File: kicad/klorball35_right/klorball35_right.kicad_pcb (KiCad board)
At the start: 2 copper layers, 138.1 x 106.1 mm, 26 parts, among them J1 TRRS, J2 Conn_01x07, SW1 SW_Push, SW11 SW_Push, SW12 SW_Push, SW13 SW_Push, SW14 SW_Push, SW15 SW_Push, SW16 SW_Push, SW17 SW_Push, SW18 SW_Push, SW2 SW_Push, SW3 SW_Push, SW4 SW_Push, SW5 SW_Push, SW6 SW_Push, SW7 SW_Push, SW8 SW_Push, SW9 SW_Push, U1 Helios

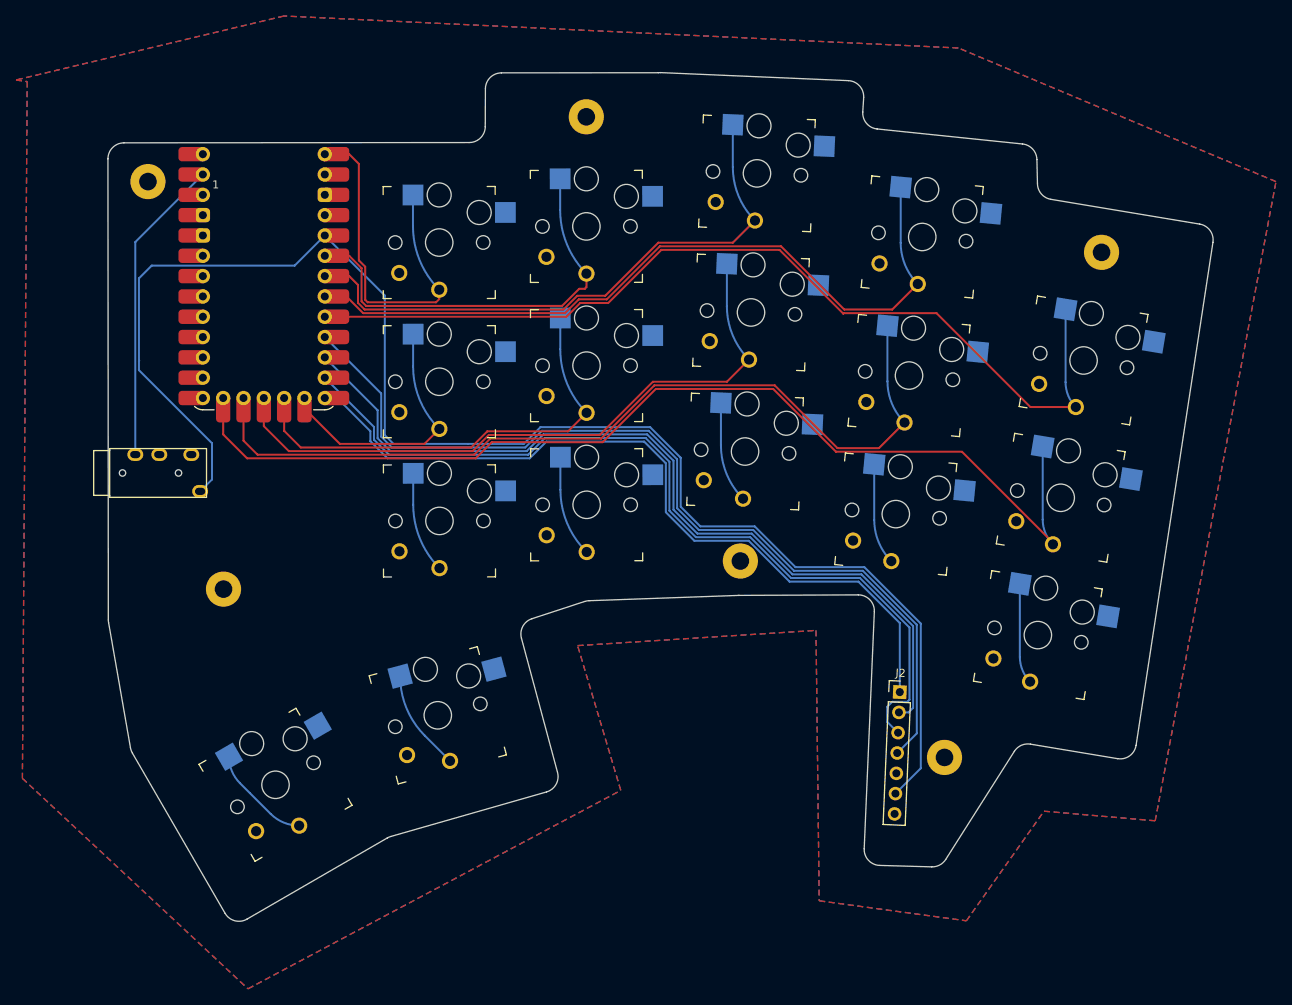
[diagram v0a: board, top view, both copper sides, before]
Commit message: finishing right, start of gerbers
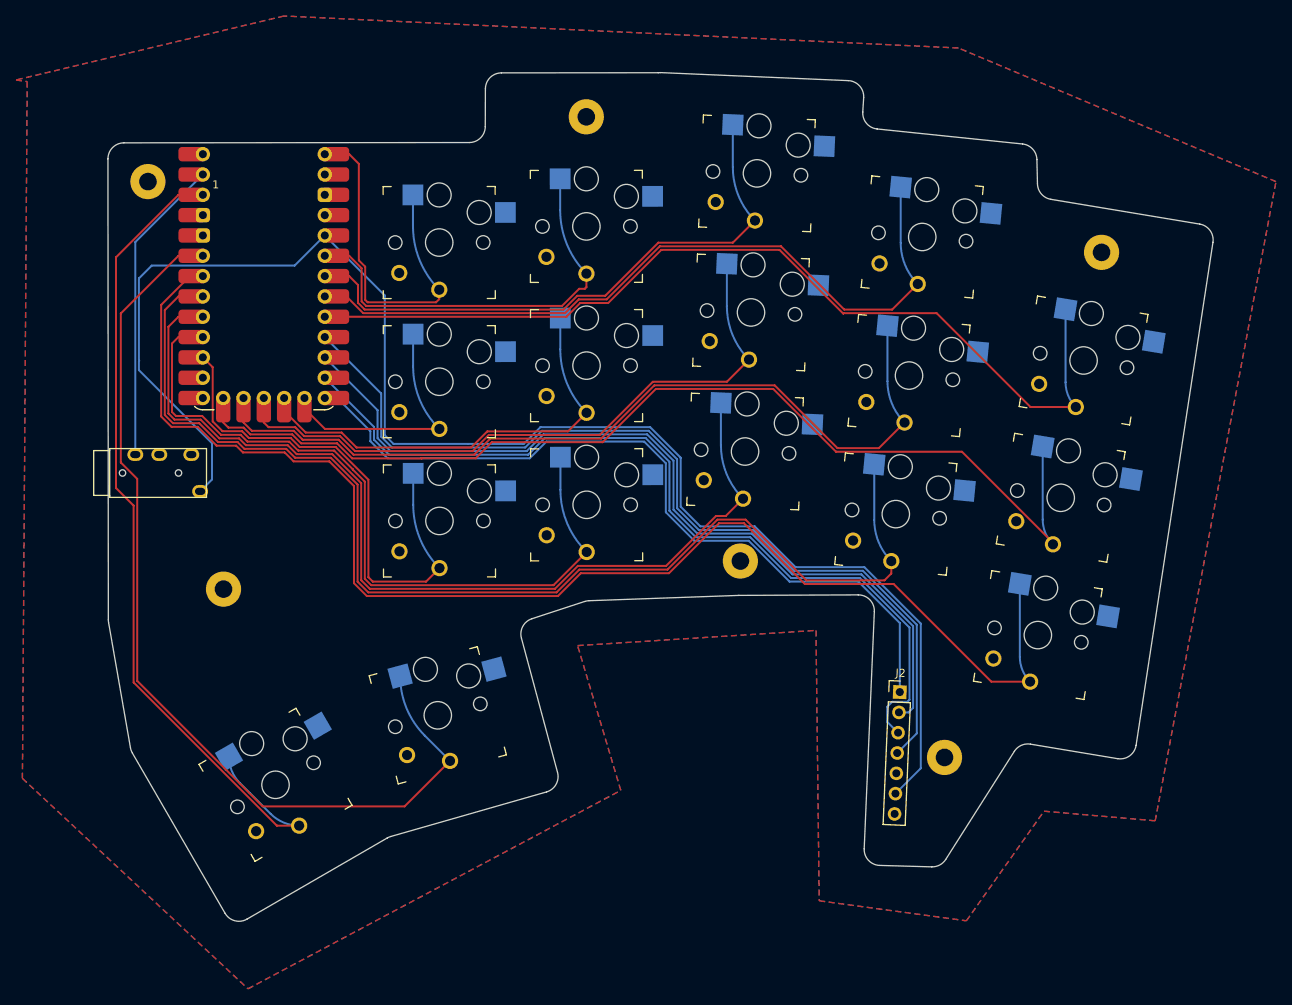
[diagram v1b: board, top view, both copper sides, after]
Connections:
- U1 pad 11: /INDEX_THUMB -> unconnected-(U1-P8-Pad11)
- U1 pad 12: /INNER_THUMB -> unconnected-(U1-P9-Pad12)_1
- U1 pad 2: unconnected-(U1-P1-Pad2)_1 -> /INNER_THUMB
- U1 pad 5: unconnected-(U1-P2-Pad5)_1 -> /INDEX_THUMB
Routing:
- net /PINKY_BOTTOM: track 12.5 -> 168.9 mm
- net /RING_BOTTOM: track 12.6 -> 145.9 mm
- net /MIDDLE_BOTTOM: track 12.7 -> 119.7 mm
- net /INDEX_THUMB: track 12.7 -> 119.4 mm
- net /INNER_THUMB: track 13.0 -> 108.0 mm
- net /INDEX_BOTTOM: track 12.7 -> 93.8 mm
- net /INNER_BOTTOM: track 12.7 -> 65.7 mm
- net /INNER_HOME: track 32.2 -> 30.6 mm
- net /INDEX_HOME: track 55.9 -> 54.5 mm
- net /RING_HOME: track 108.2 -> 106.9 mm
- net /PINKY_HOME: track 132.5 -> 131.6 mm
